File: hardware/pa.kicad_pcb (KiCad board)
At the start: 2 copper layers, 100 x 80 mm, 95 parts, among them J1 Conn_Coaxial, J11 RXSupply, J2 FromRX, J3 Barrel_Jack_Switch, J6 RX-HF, J7 TX-HF, K1 G6S-2, K2 G6S-2, K3 G6S-2, K4 G6S-2, Q1 2N3904, Q10 2N3904, Q11 BS170, Q2 2N3904, Q3 2N3904, Q4 BS170, Q5 BD140-16, Q6 BS170, Q7 BS170, Q8 BS170, Q9 BS170, T1 8+8@FT37-43, U1 74HCT00

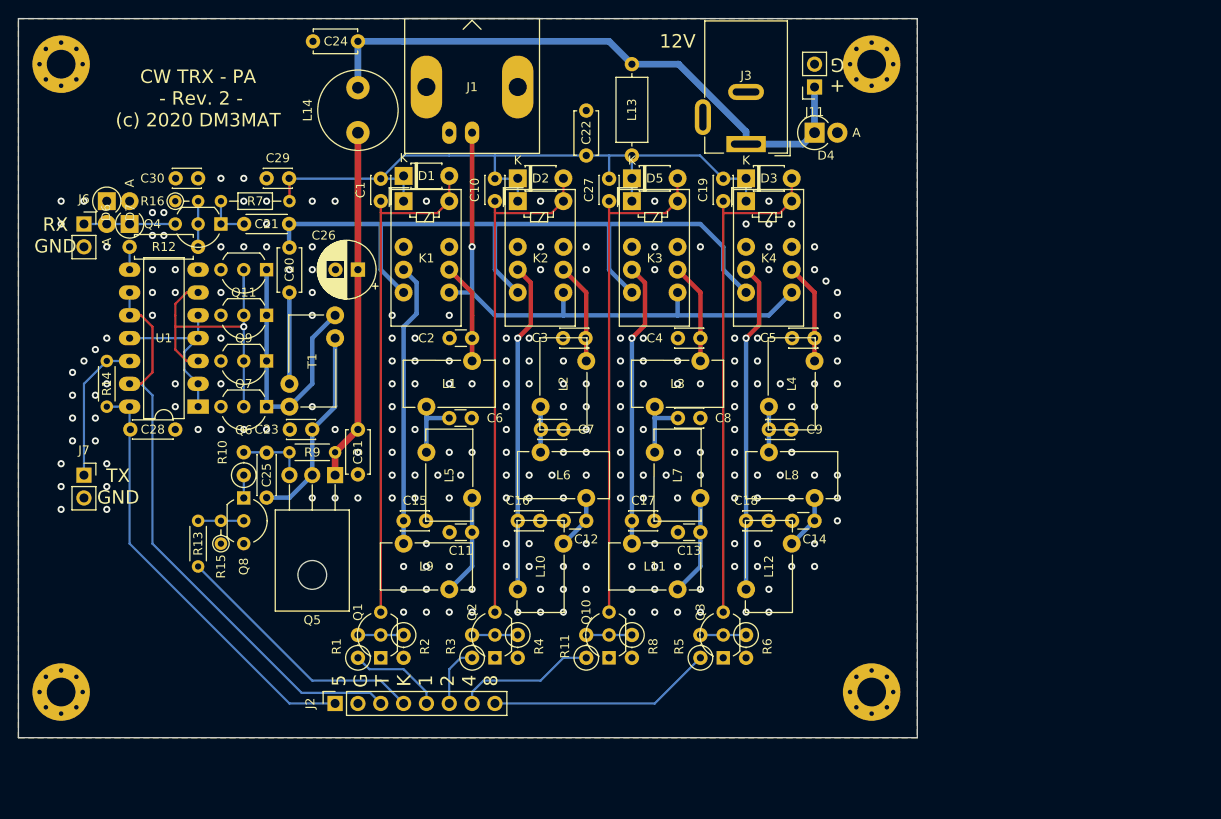
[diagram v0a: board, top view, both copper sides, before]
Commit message: Fixed docs.
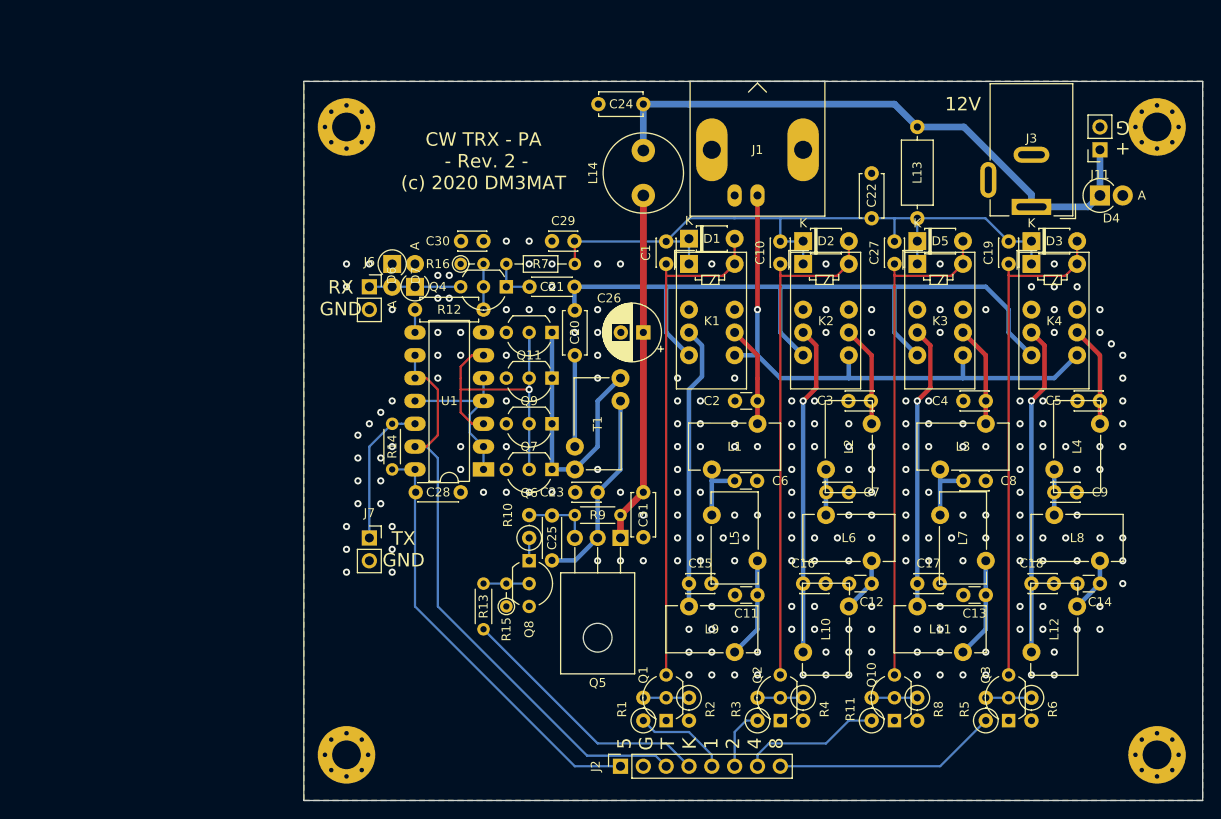
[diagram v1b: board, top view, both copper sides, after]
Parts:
- moved C16 32.5 mm to (157.3, 112.9)
- moved C24 32.5 mm to (134.5, 59.5)
- moved C25 32.5 mm to (129.4, 110.3)
- moved C26 32.5 mm to (139.5, 84.9)
- moved C29 32.5 mm to (129.4, 74.8)
- moved C31 32.5 mm to (139.5, 107.7)
- moved D2 32.5 mm to (157.3, 74.8)
- moved K2 32.5 mm to (157.3, 77.3)
- moved L14 32.5 mm to (139.5, 69.7)
- moved Q11 32.5 mm to (129.4, 84.9)
- moved Q6 32.5 mm to (129.4, 100.2)
- moved Q7 32.5 mm to (129.4, 95.1)
- moved Q9 32.5 mm to (129.4, 90.0)
- moved R1 32.5 mm to (139.5, 128.1)
- moved R4 32.5 mm to (157.3, 125.6)
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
